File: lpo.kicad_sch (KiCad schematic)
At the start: 7 parts, among them J10 Conn_01x02, Q1 AO3400A

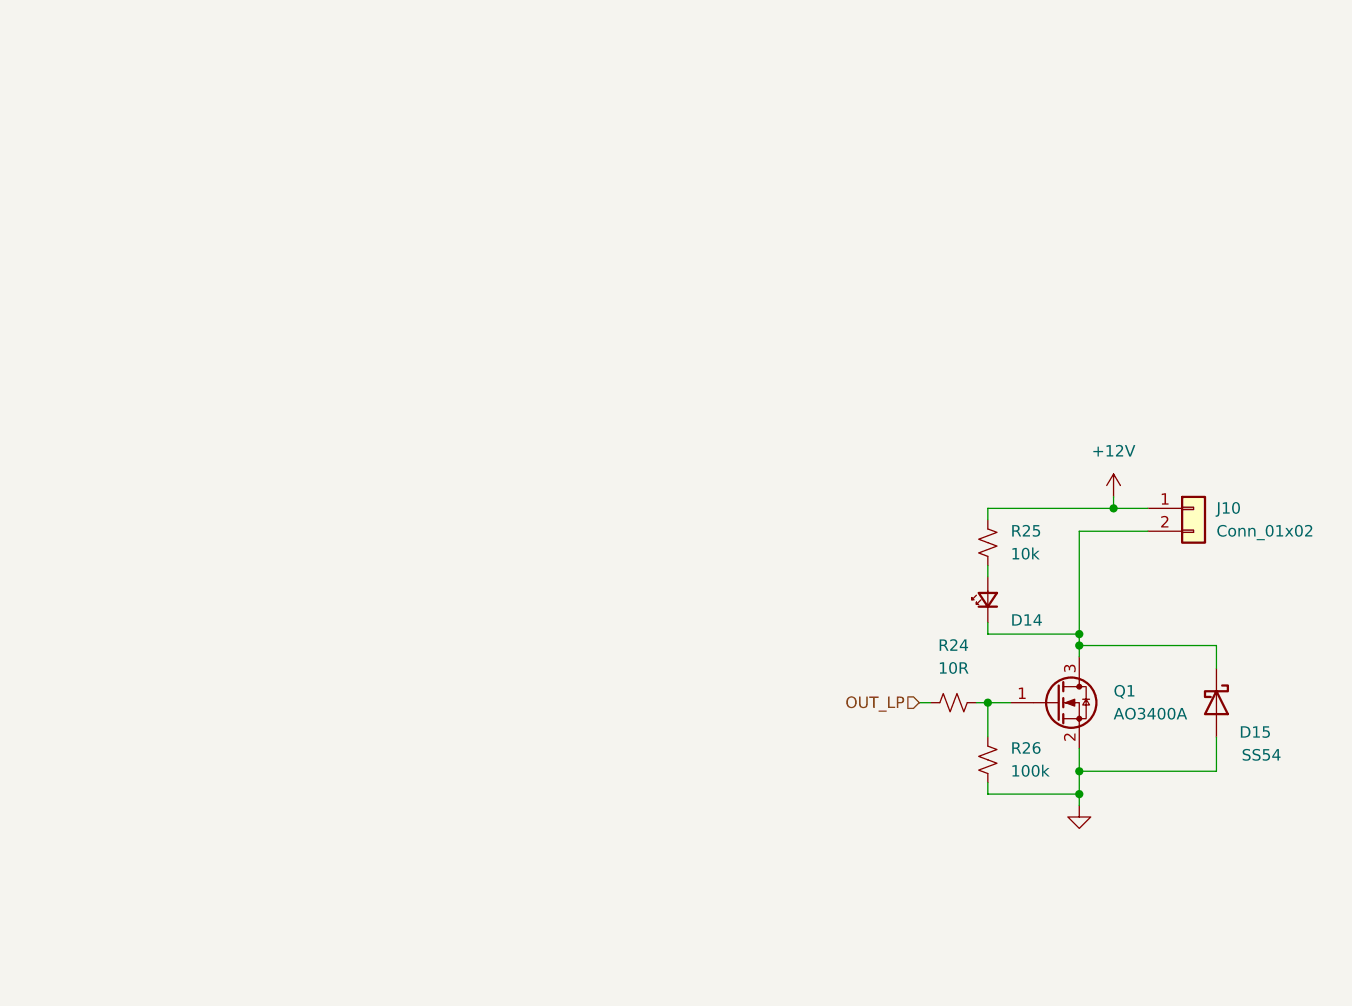
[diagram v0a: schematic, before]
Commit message: ???
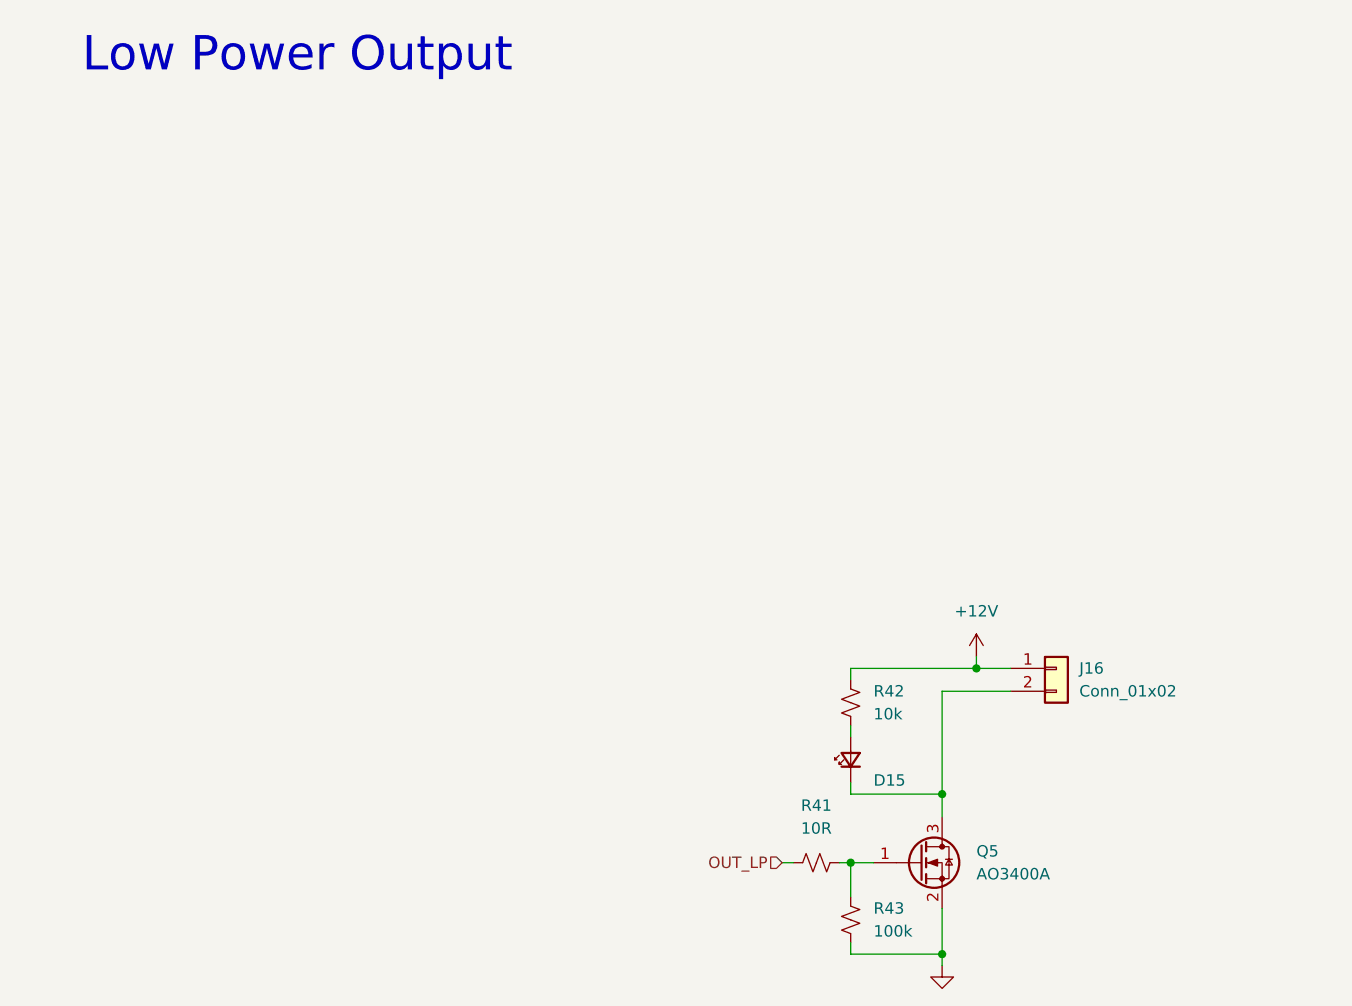
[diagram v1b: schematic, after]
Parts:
- removed D14: LED_Small, APRLPrints:LED_0603, symbol Device:LED_Small
- removed D15: SS54, Diode_SMD:D_SMA, symbol Diode:SS38
- removed J10: Conn_01x02, Connector_Molex:Molex_Micro-Fit_3.0_43650-0215_1x02_P3.00mm_Vertical, symbol Connector_Generic:Conn_01x02
- removed Q1: AO3400A, Package_TO_SOT_SMD:SOT-23, symbol Transistor_FET:AO3400A
- removed R24: 10R, APRLPrints:R_0603, symbol Device:R_Small_US
- removed R25: 10k, APRLPrints:R_0603, symbol Device:R_Small_US
- removed R26: 100k, APRLPrints:R_0603, symbol Device:R_Small_US
- added D15: LED_Small, APRLPrints:LED_0603, symbol Device:LED_Small
- added J16: Conn_01x02, Connector_Molex:Molex_Micro-Fit_3.0_43650-0215_1x02_P3.00mm_Vertical, symbol Connector_Generic:Conn_01x02
- added Q5: AO3400A, Package_TO_SOT_SMD:SOT-23, symbol Transistor_FET:AO3400A
- added R41: 10R, APRLPrints:R_0603, symbol Device:R_Small_US
- added R42: 10k, APRLPrints:R_0603, symbol Device:R_Small_US
- added R43: 100k, APRLPrints:R_0603, symbol Device:R_Small_US
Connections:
- net +12V: now also J16.1 (Pin_1), R42.1
- net GND: now also Q5.2 (S), R43.1
- net OUT_LP: now also R41.1
- new net: D15.1 (K), J16.2 (Pin_2), Q5.3 (D)
- new net: D15.2 (A), R42.2
- new net: Q5.1 (G), R41.2, R43.2
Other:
- note added: "Low Power Output"
